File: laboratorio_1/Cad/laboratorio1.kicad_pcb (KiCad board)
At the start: 2 copper layers, 93.5 x 96 mm, 35 parts, among them J5 Output, J6 VA1, J7 Vin, J8 Vout, J9 Masa, U1 TL084, U2 TL084, j1 Vdd, j2 Vss, j3 GND, j4 Input

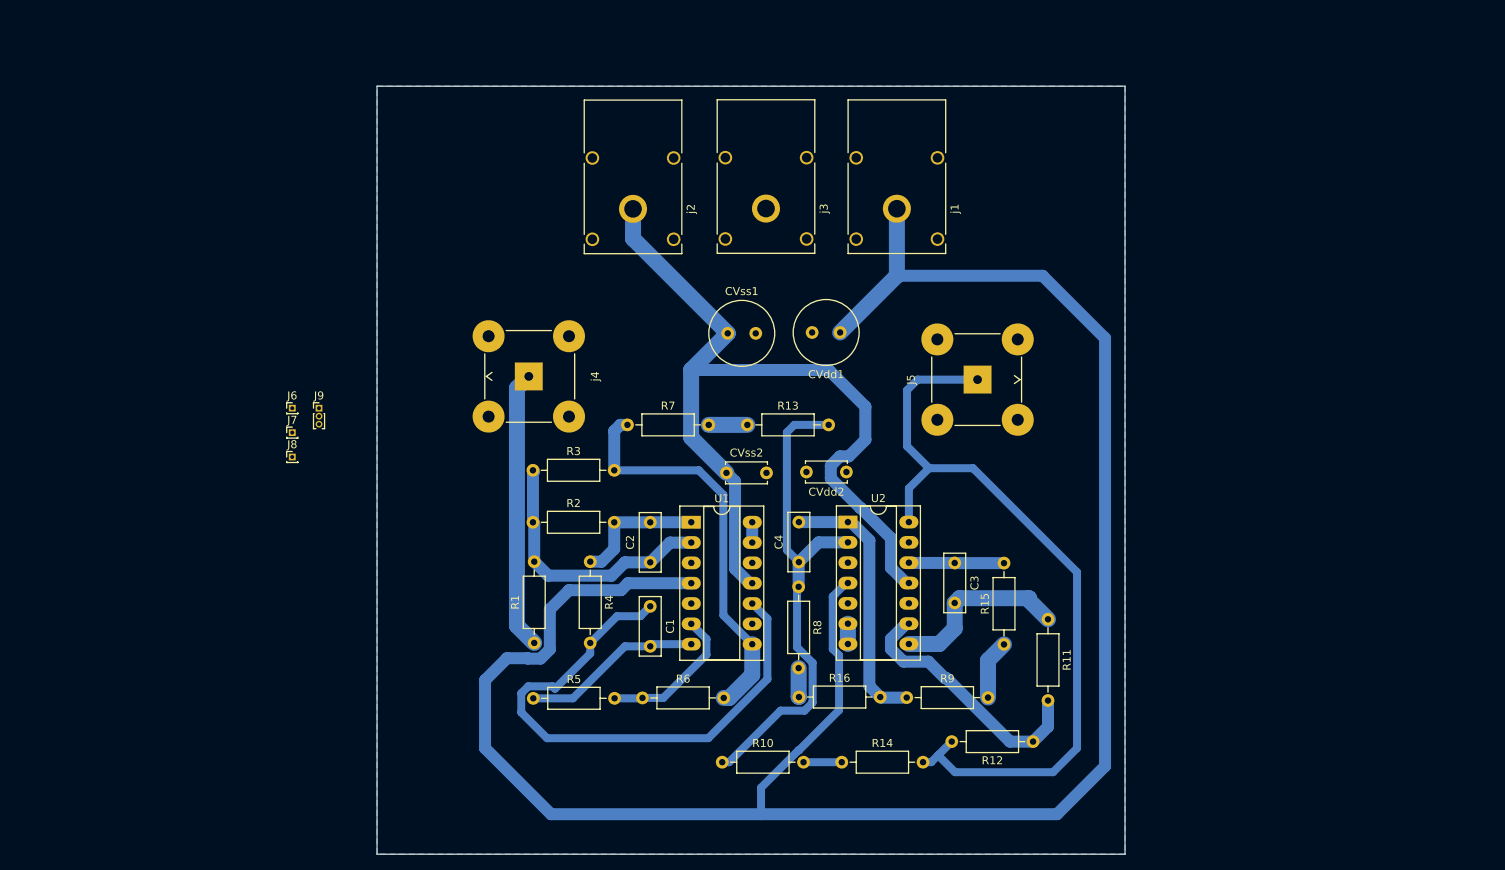
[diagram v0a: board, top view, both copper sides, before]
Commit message: actualizo desde linux
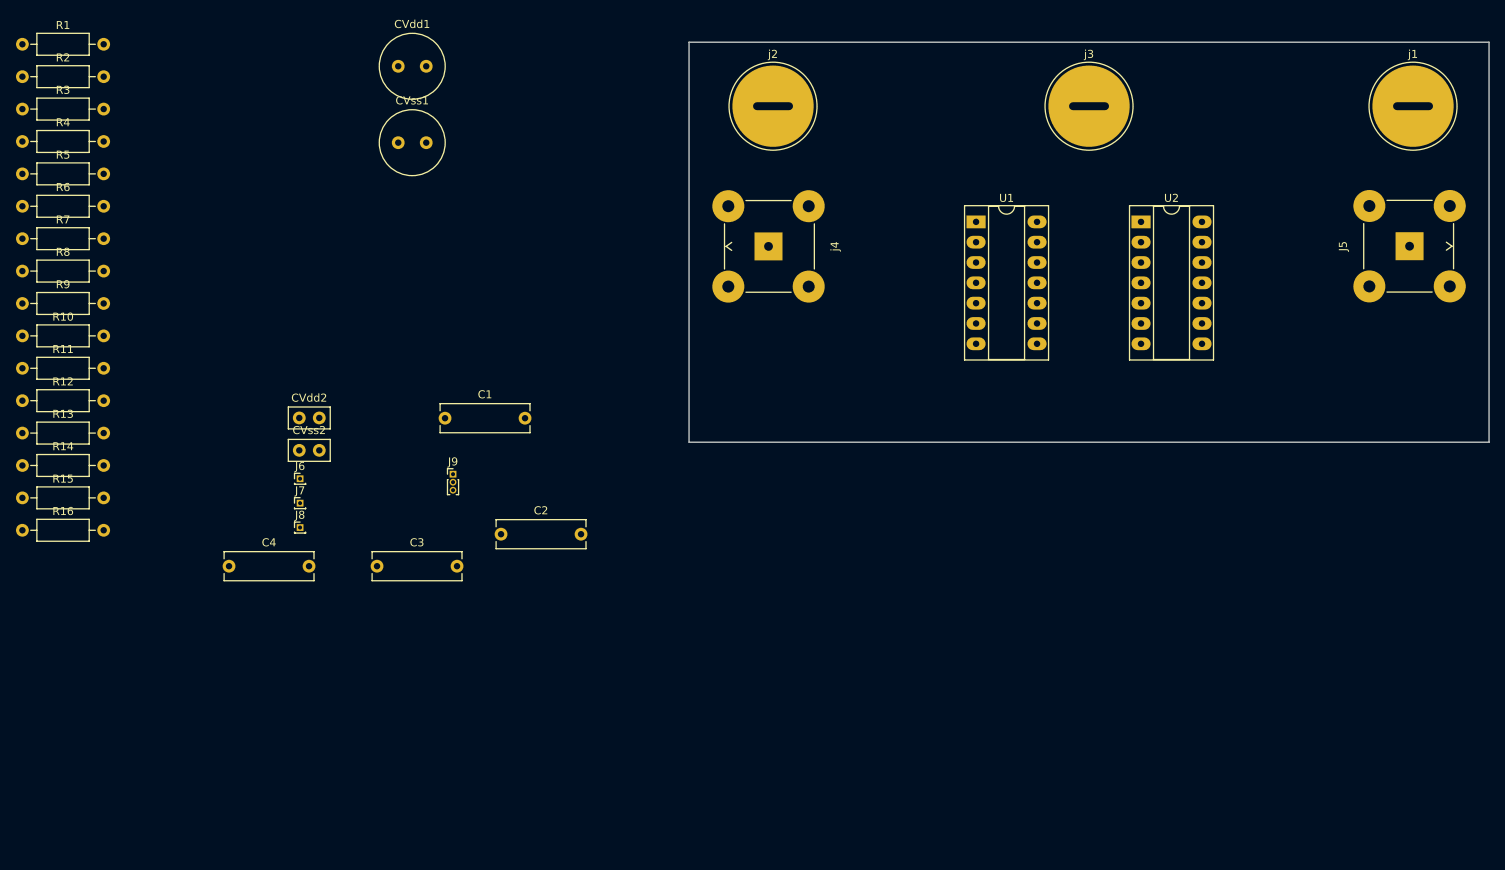
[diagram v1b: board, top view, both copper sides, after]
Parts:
- C1, C2, C3, C4: footprint Capacitor_THT:C_Rect_L7.2mm_W2.5mm_P5.00mm_FKS2_FKP2_MKS2_MKP2 -> Capacitor_THT:C_Rect_L11.0mm_W3.4mm_P10.00mm_MKT
- CVdd2, CVss2: footprint Capacitor_THT:C_Disc_D5.0mm_W2.5mm_P5.00mm -> Capacitor_THT:C_Disc_D5.0mm_W2.5mm_P2.50mm
- j1: footprint Connector:Banana_Cliff_FCR7350R_S16N-PC_Horizontal -> Connector:Banana_Jack_1Pin
- j2: footprint Connector:Banana_Cliff_FCR7350L_S16N-PC_Horizontal -> Connector:Banana_Jack_1Pin
- j3: footprint Connector:Banana_Cliff_FCR7350G_S16N-PC_Horizontal -> Connector:Banana_Jack_1Pin
- moved R12 133.3 mm to (51.7, 94.8), turned to 0 degrees
- moved R11 132.0 mm to (51.7, 90.8), turned to 0 degrees
- moved R15 124.1 mm to (51.7, 107.0), turned to 0 degrees
- moved R9 121.0 mm to (51.7, 82.7)
- moved R14 108.9 mm to (51.7, 102.9)
- moved R8 104.7 mm to (51.7, 78.6), turned to 0 degrees
- moved R10 102.4 mm to (51.7, 86.7)
- moved R16 99.3 mm to (51.7, 111.0)
- moved R6 98.9 mm to (51.7, 70.5)
- moved R1 98.5 mm to (51.7, 50.3), turned to 0 degrees
- moved R5 91.5 mm to (51.7, 66.5)
- moved R13 90.6 mm to (51.7, 98.9)
- moved R4 88.3 mm to (51.7, 62.4), turned to 0 degrees
- moved R2 84.7 mm to (51.7, 54.3)
- moved R7 79.1 mm to (51.7, 74.6)
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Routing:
- net Net-(U1E-V+): track 261.0 -> 0.00 mm
- net Net-(U1E-V-): track 109.4 -> 0.00 mm
- net Net-(J5-In): track 98.1 -> 0.00 mm
- net Net-(U1C-+): track 69.8 -> 0.00 mm
- net Net-(U2A--): track 62.4 -> 0.00 mm
- net Net-(J6-Pin_1): track 50.6 -> 0.00 mm
- net Net-(J7-Pin_1): track 34.8 -> 0.00 mm
- net Net-(U1A--): track 33.8 -> 0.00 mm
- net Net-(C4-Pad2): track 33.2 -> 0.00 mm
- net Net-(U2C--): track 32.7 -> 0.00 mm
- net Net-(C3-Pad2): track 22.9 -> 0.00 mm
- net Net-(C1-Pad2): track 22.6 -> 0.00 mm
- net Net-(U1B--): track 18.4 -> 0.00 mm
- net Net-(C2-Pad2): track 16.6 -> 0.00 mm
- net Net-(U2D-+): track 11.9 -> 0.00 mm
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- removed copper zone on B.Cu, net GND
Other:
- board size 93.5 x 96 mm -> 100 x 50 mm
- board text removed: "R5"
